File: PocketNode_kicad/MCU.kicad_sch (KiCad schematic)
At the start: 1 part, among them U3 ESP32-S3-WROOM-1-N16R8

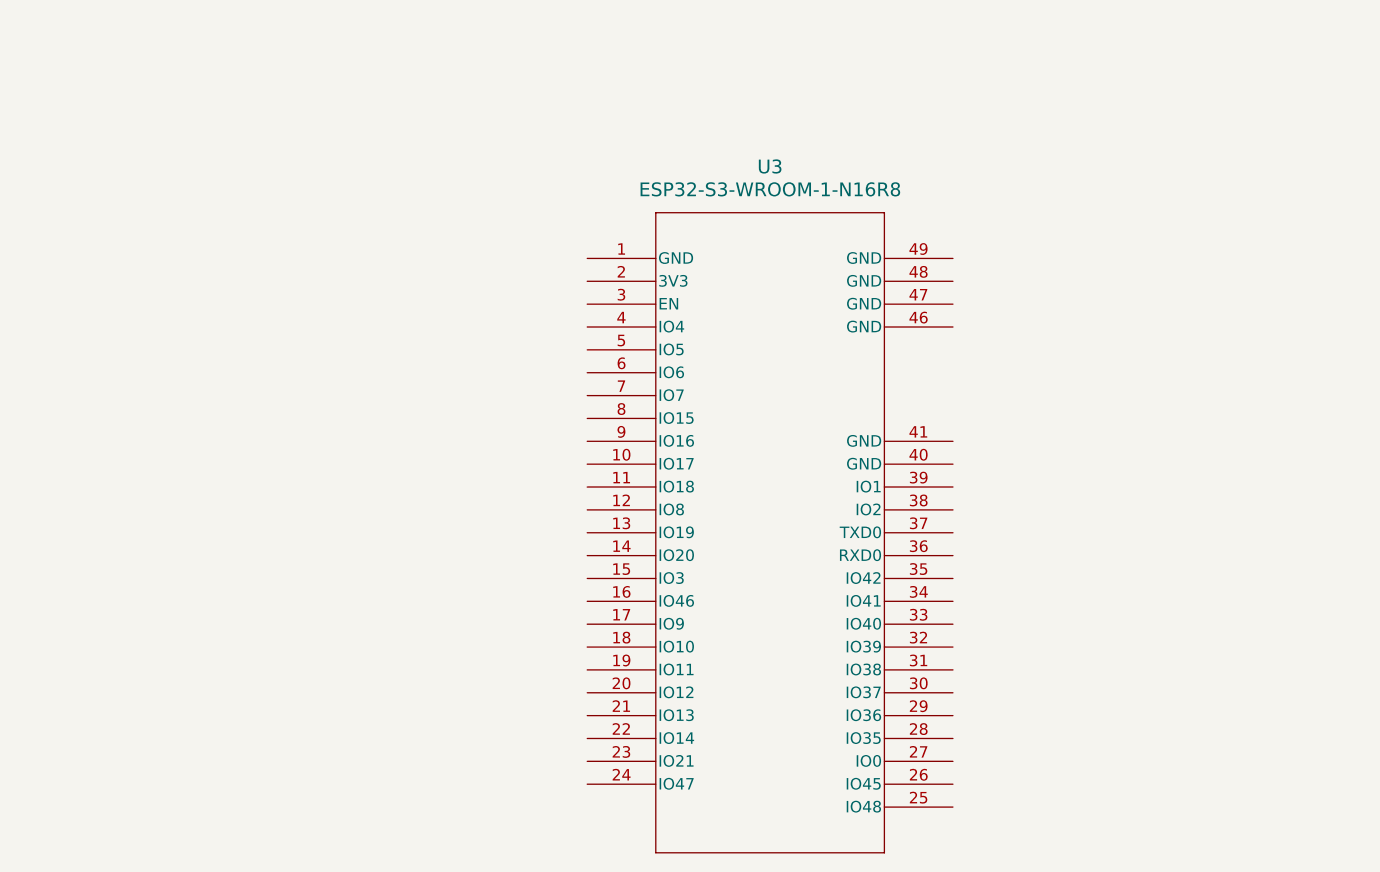
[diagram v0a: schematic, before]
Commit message: update2
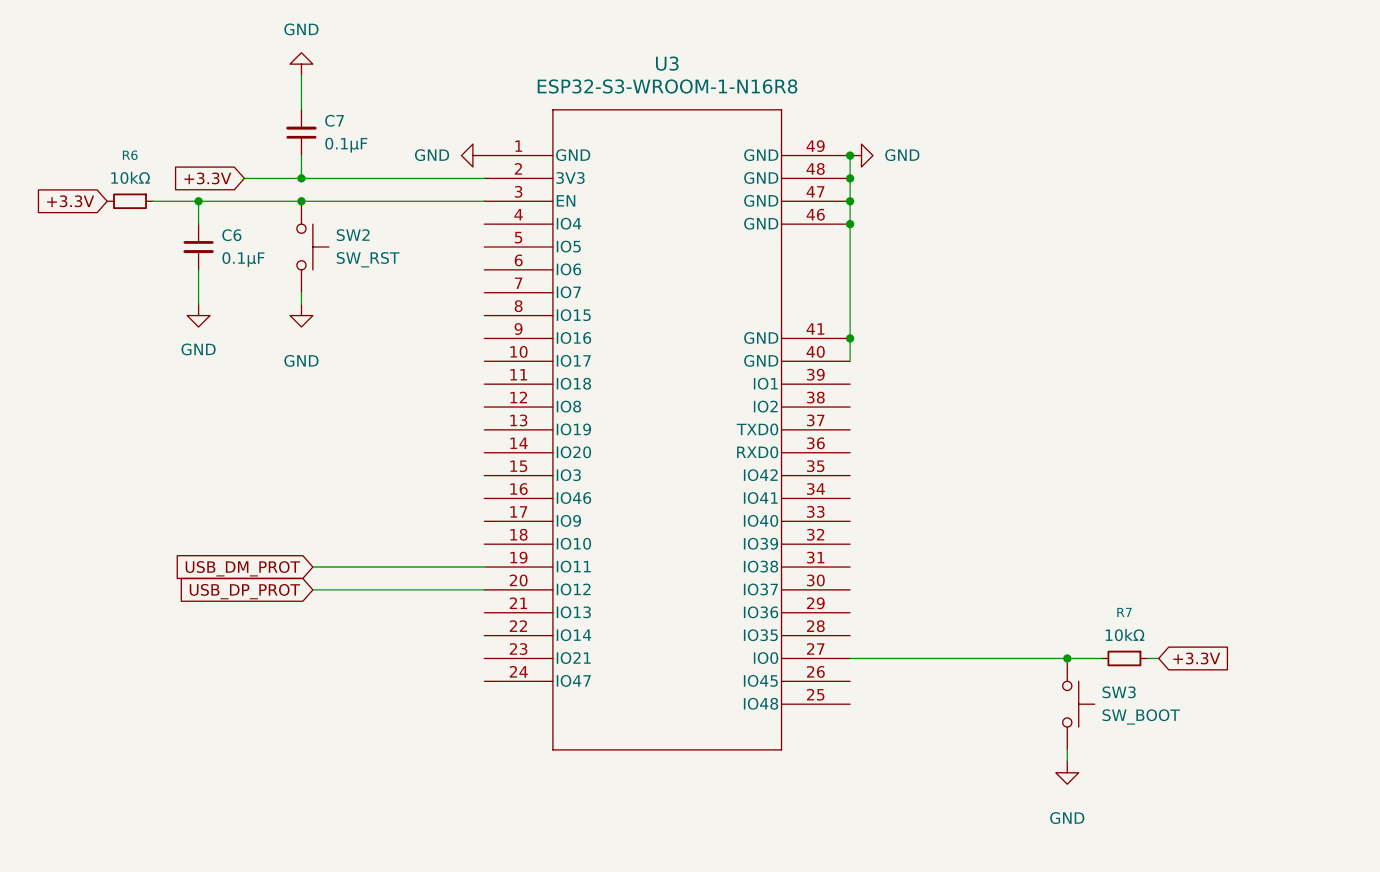
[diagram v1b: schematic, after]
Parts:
- added C6, C7: 0.1μF, symbol Device:C_Small
- added R6, R7: 10kΩ, symbol Device:R_Small
- added SW2: SW_RST, symbol Switch:SW_Push
- added SW3: SW_BOOT, symbol Switch:SW_Push
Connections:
- net GND: now reaches U3.1 (GND)
- net GND: now also U3.40 (GND), U3.41 (GND), U3.46 (GND), U3.47 (GND), U3.48 (GND), U3.49 (GND), C6.2, C7.2, SW2.2, SW3.2
- net USB_DM_PROT: now reaches U3.19 (IO11)
- net +3.3V: now reaches U3.2 (3V3)
- net +3.3V: now also C7.1, R6.2, R7.1
- net USB_DP_PROT: now reaches U3.20 (IO12)
- net at U3.27 (IO0): now also R7.2, SW3.1
- net at U3.3 (EN): now also C6.1, R6.1, SW2.1
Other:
- moved on the sheet: U3

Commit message: update3
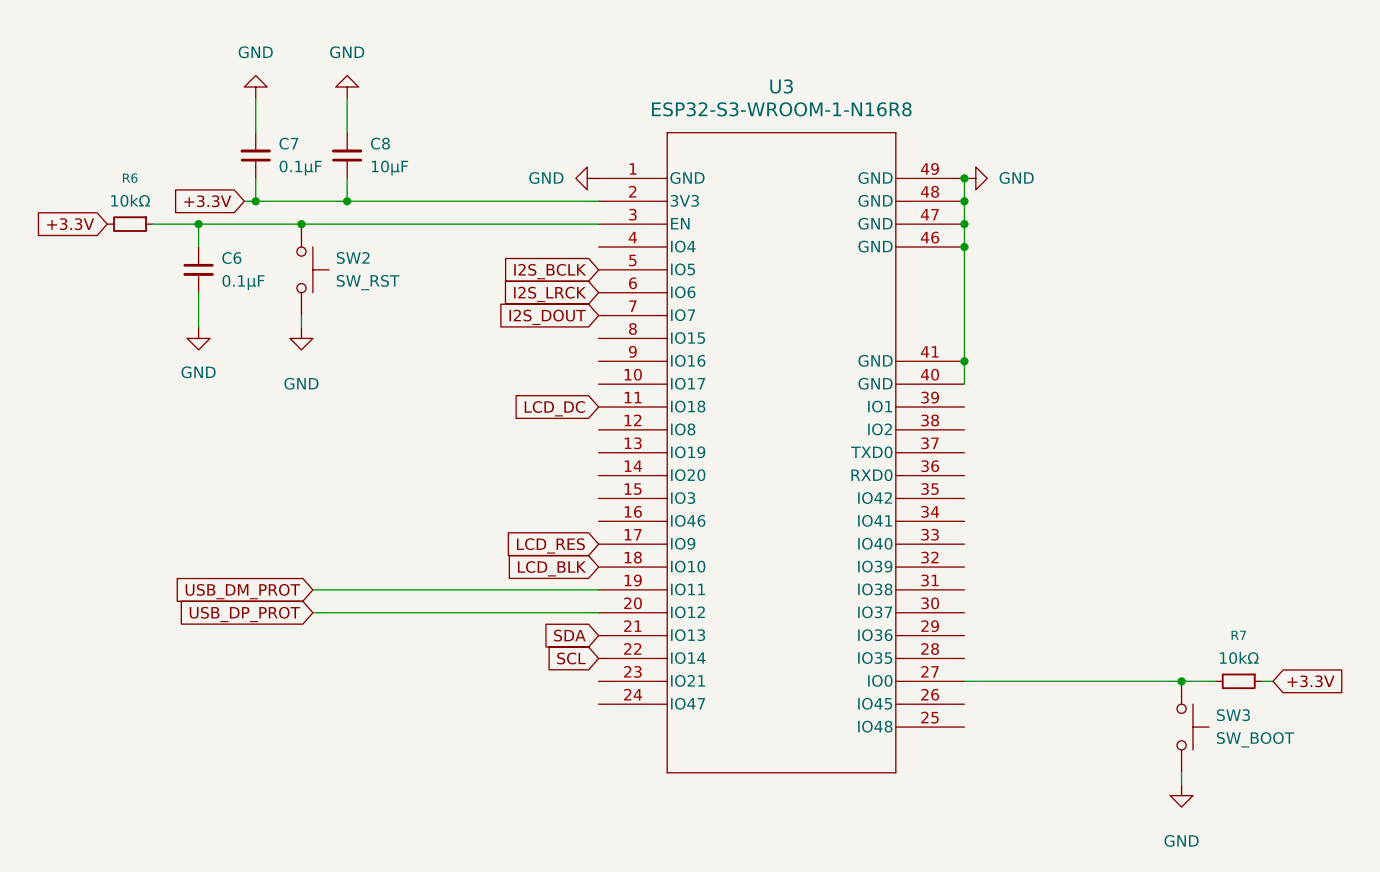
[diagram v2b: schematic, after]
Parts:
- added C8: 10μF, symbol Device:C_Small
- U3: footprint ESP32-S3-WROOM-1_EXP -> Library:ESP32-S3-WROOM-1_EXP
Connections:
- net +3.3V: now also C8.1
- net GND: now also C8.2
- net LCD_DC: now reaches U3.11 (IO18)
- net LCD_RES: now reaches U3.17 (IO9)
- net LCD_BLK: now reaches U3.18 (IO10)
- net SDA: now reaches U3.21 (IO13)
- net SCL: now reaches U3.22 (IO14)
- net I2S_BCLK: now reaches U3.5 (IO5)
- net I2S_LRCK: now reaches U3.6 (IO6)
- net I2S_DOUT: now reaches U3.7 (IO7)
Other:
- moved on the sheet: C6, C7, R6, R7, SW2, SW3, U3

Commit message: update4
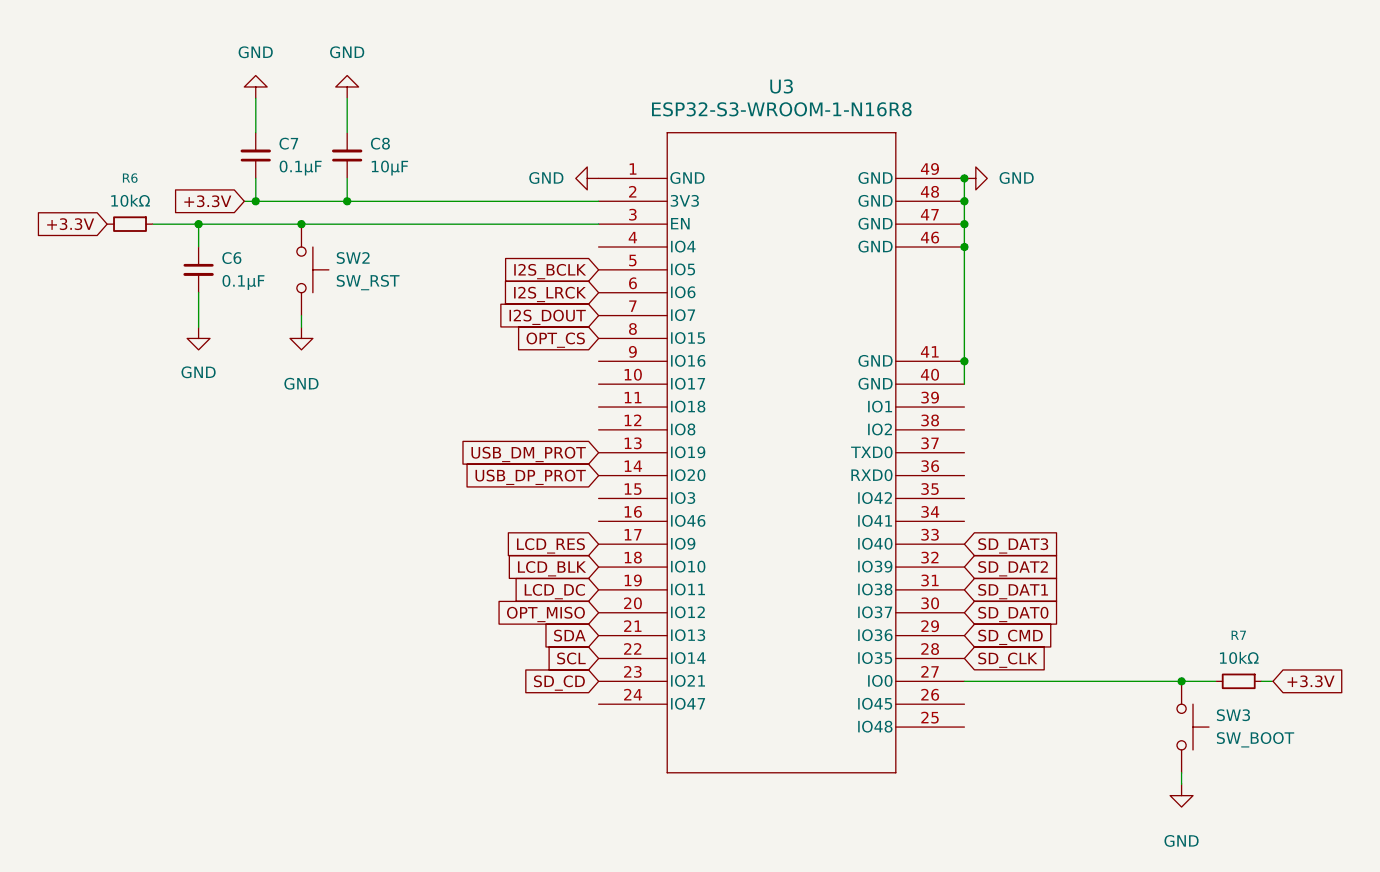
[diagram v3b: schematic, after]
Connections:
- net LCD_DC: now also U3.19 (IO11); no longer U3.11 (IO18)
- net USB_DM_PROT: now also U3.13 (IO19); no longer U3.19 (IO11)
- net USB_DP_PROT: now also U3.14 (IO20); no longer U3.20 (IO12)
- net SD_CD: now reaches U3.23 (IO21)
- net SD_CLK: now reaches U3.28 (IO35)
- net SD_CMD: now reaches U3.29 (IO36)
- net SD_DAT0: now reaches U3.30 (IO37)
- net SD_DAT1: now reaches U3.31 (IO38)
- net SD_DAT2: now reaches U3.32 (IO39)
- net SD_DAT3: now reaches U3.33 (IO40)
- net OPT_CS: now reaches U3.8 (IO15)
- new net OPT_MISO: U3.20 (IO12)
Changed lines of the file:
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@@
-	(wire
-		(pts
-			(xy 96.52 74.93) (xy 128.27 74.93)
-		)
-		(stroke
-			(width 0)
-			(type default)
-		)
-	)
 	(wire
 		(pts
@@
 	(wire
 		(pts
-			(xy 96.52 77.47) (xy 128.27 77.47)
-		)
-		(stroke
-			(width 0)
-			(type default)
-		)
-	)
-	(wire
-		(pts
 			(xy 100.33 20.32) (xy 100.33 24.13)
 		)
@@
 		)
 	)
+	(global_label "SD_CD"
+		(shape input)
+		(at 128.27 85.09 180)
+		(fields_autoplaced yes)
+		(effects
+			(font
+				(size 1.27 1.27)
+			)
+			(justify right)
+		)
+		(property "Intersheetrefs" "${INTERSHEET_REFS}"
+			(at 119.2977 85.09 0)
+			(effects
+				(font
+					(size 1.27 1.27)
+				)
+				(justify right)
+				(hide yes)
+			)
+		)
+	)
+	(global_label "SD_CMD"
+		(shape input)
+		(at 168.91 80.01 0)
+		(fields_autoplaced yes)
+		(effects
+			(font
+				(size 1.27 1.27)
+			)
+			(justify left)
+		)
+		(property "Intersheetrefs" "${INTERSHEET_REFS}"
+			(at 179.3337 80.01 0)
+			(effects
+				(font
+					(size 1.27 1.27)
+				)
+				(justify left)
+				(hide yes)
+			)
+		)
+	)
+	(global_label "SD_CLK"
+		(shape input)
+		(at 168.91 82.55 0)
+		(fields_autoplaced yes)
+		(effects
+			(font
+				(size 1.27 1.27)
+			)
+			(justify left)
+		)
+		(property "Intersheetrefs" "${INTERSHEET_REFS}"
+			(at 178.9104 82.55 0)
+			(effects
+				(font
+					(size 1.27 1.27)
+				)
+				(justify left)
+				(hide yes)
+			)
+		)
+	)
 	(global_label "+3.3V"
 		(shape input)
@@
 		)
 	)
+	(global_label "SD_DAT3"
+		(shape input)
+		(at 168.91 69.85 0)
+		(fields_autoplaced yes)
+		(effects
+			(font
+				(size 1.27 1.27)
+			)
+			(justify left)
+		)
+		(property "Intersheetrefs" "${INTERSHEET_REFS}"
+			(at 179.878 69.85 0)
+			(effects
+				(font
+					(size 1.27 1.27)
+				)
+				(justify left)
+				(hide yes)
+			)
+		)
+	)
+	(global_label "OPT_MISO"
+		(shape input)
+		(at 128.27 77.47 180)
+		(fields_autoplaced yes)
+		(effects
+			(font
+				(size 1.27 1.27)
+			)
+			(justify right)
+		)
+		(property "Intersheetrefs" "${INTERSHEET_REFS}"
+			(at 116.1529 77.47 0)
+			(effects
+				(font
+					(size 1.27 1.27)
+				)
+				(justify right)
+				(hide yes)
+			)
+		)
+	)
+	(global_label "SD_DAT2"
+		(shape input)
+		(at 168.91 72.39 0)
+		(fields_autoplaced yes)
+		(effects
+			(font
+				(size 1.27 1.27)
+			)
+			(justify left)
+		)
+		(property "Intersheetrefs" "${INTERSHEET_REFS}"
+			(at 179.878 72.39 0)
+			(effects
+				(font
+					(size 1.27 1.27)
+				)
+				(justify left)
+				(hide yes)
+			)
+		)
+	)
+	(global_label "OPT_CS"
+		(shape input)
+		(at 128.27 46.99 180)
+		(fields_autoplaced yes)
+		(effects
+			(font
+				(size 1.27 1.27)
+			)
+			(justify right)
+		)
+		(property "Intersheetrefs" "${INTERSHEET_REFS}"
+			(at 118.2696 46.99 0)
+			(effects
+				(font
+					(size 1.27 1.27)
+				)
+				(justify right)
+				(hide yes)
+			)
+		)
+	)
+	(global_label "SD_DAT1"
+		(shape input)
+		(at 168.91 74.93 0)
+		(fields_autoplaced yes)
+		(effects
+			(font
+				(size 1.27 1.27)
+			)
+			(justify left)
+		)
+		(property "Intersheetrefs" "${INTERSHEET_REFS}"
+			(at 179.878 74.93 0)
+			(effects
+				(font
+					(size 1.27 1.27)
+				)
+				(justify left)
+				(hide yes)
+			)
+		)
+	)
 	(global_label "I2S_BCLK"
 		(shape input)
@@
 	(global_label "LCD_DC"
 		(shape input)
-		(at 128.27 54.61 180)
-		(fields_autoplaced yes)
-		(effects
-			(font
-				(size 1.27 1.27)
-			)
-			(justify right)
-		)
-		(property "Intersheetrefs" "${INTERSHEET_REFS}"
-			(at 118.2091 54.61 0)
+		(at 128.27 74.93 180)
+		(fields_autoplaced yes)
+		(effects
+			(font
+				(size 1.27 1.27)
+			)
+			(justify right)
+		)
+		(property "Intersheetrefs" "${INTERSHEET_REFS}"
+			(at 118.2091 74.93 0)
 			(effects
 				(font
@@
 		)
 	)
+	(global_label "SD_DAT0"
+		(shape input)
+		(at 168.91 77.47 0)
+		(fields_autoplaced yes)
+		(effects
+			(font
+				(size 1.27 1.27)
+			)
+			(justify left)
+		)
+		(property "Intersheetrefs" "${INTERSHEET_REFS}"
+			(at 179.878 77.47 0)
+			(effects
+				(font
+					(size 1.27 1.27)
+				)
+				(justify left)
+				(hide yes)
+			)
+		)
+	)
 	(global_label "SDA"
 		(shape input)
@@
 	(global_label "USB_DM_PROT"
 		(shape input)
-		(at 96.52 74.93 180)
-		(fields_autoplaced yes)
-		(effects
-			(font
-				(size 1.27 1.27)
-			)
-			(justify right)
-		)
-		(property "Intersheetrefs" "${INTERSHEET_REFS}"
-			(at 80.2301 74.93 0)
+		(at 128.27 59.69 180)
+		(fields_autoplaced yes)
+		(effects
+			(font
+				(size 1.27 1.27)
+			)
+			(justify right)
+		)
+		(property "Intersheetrefs" "${INTERSHEET_REFS}"
+			(at 111.9801 59.69 0)
 			(effects
 				(font
@@
 	(global_label "USB_DP_PROT"
 		(shape input)
-		(at 96.52 77.47 180)
-		(fields_autoplaced yes)
-		(effects
-			(font
-				(size 1.27 1.27)
-			)
-			(justify right)
-		)
-		(property "Intersheetrefs" "${INTERSHEET_REFS}"
-			(at 80.4115 77.47 0)
-			(effects
-				(font
+		(at 128.27 62.23 180)
+		(fields_autoplaced yes)
+		(effects
+			(font
+				(size 1.27 1.27)
+			)
+			(justify right)
+		)
+		(property "Intersheetrefs" "${INTERSHEET_REFS}"
+			(at 112.1615 62.23 0)
+			(effects
+				(font
